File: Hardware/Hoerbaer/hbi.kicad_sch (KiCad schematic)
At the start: 50 parts, among them J10 LEDS, J11 LEDS, J6 BUTTONS, J7 BUTTONS, J8 BUTTONS, J9 LEDS, U2 PCF8574APWR, U3 PCF8574APWR, U4 PCF8574APWR, U5 TLC59108xPW, U6 TLC59108xPW, U7 TLC59108xPW

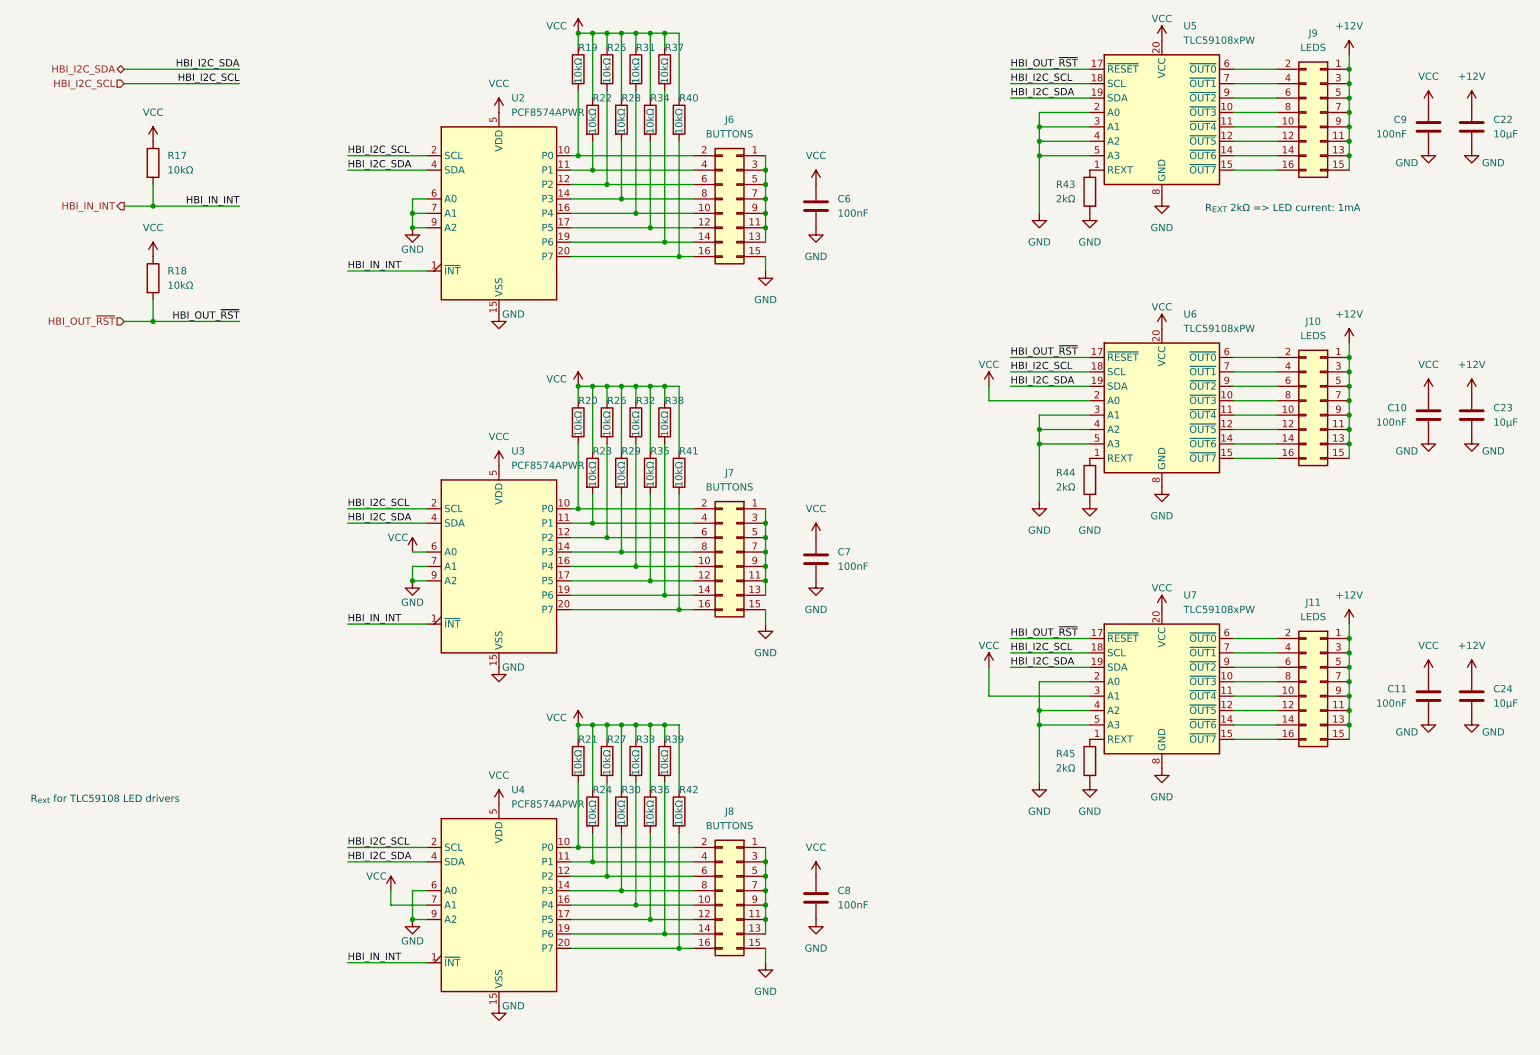
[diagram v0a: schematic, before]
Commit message: Layout drc error free
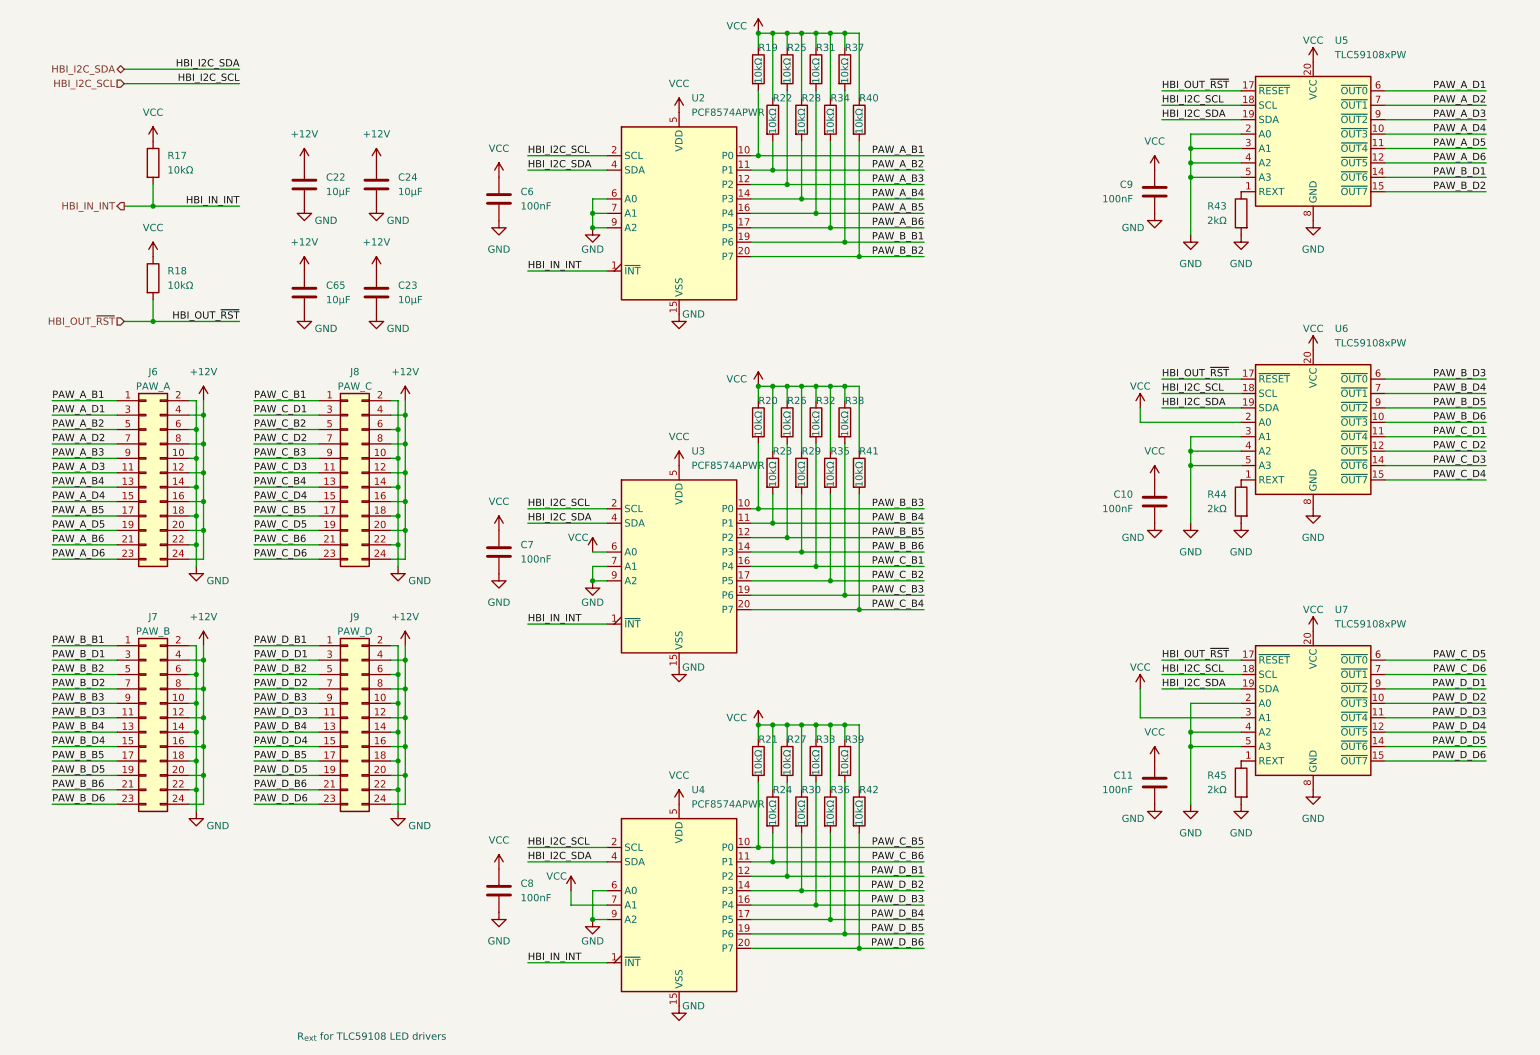
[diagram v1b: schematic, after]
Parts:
- removed J10, J11, J9: LEDS, Connector_PinHeader_2.54mm:PinHeader_2x08_P2.54mm_Vertical, symbol Connector_Generic:Conn_02x08_Odd_Even
- removed J7, J8: BUTTONS, Connector_PinHeader_2.54mm:PinHeader_2x08_P2.54mm_Vertical, symbol Connector_Generic:Conn_02x08_Odd_Even
- added C65: 10µF, Capacitor_SMD:C_0805_2012Metric, symbol Device:C
- added J7: PAW_B, Connector_PinHeader_2.54mm:PinHeader_2x12_P2.54mm_Vertical, symbol Connector_Generic:Conn_02x12_Odd_Even
- added J8: PAW_C, Connector_PinHeader_2.54mm:PinHeader_2x12_P2.54mm_Vertical, symbol Connector_Generic:Conn_02x12_Odd_Even
- added J9: PAW_D, Connector_PinHeader_2.54mm:PinHeader_2x12_P2.54mm_Vertical, symbol Connector_Generic:Conn_02x12_Odd_Even
- J6: value BUTTONS -> PAW_A; footprint Connector_PinHeader_2.54mm:PinHeader_2x08_P2.54mm_Vertical -> Connector_PinHeader_2.54mm:PinHeader_2x12_P2.54mm_Vertical; symbol Connector_Generic:Conn_02x08_Odd_Even -> Connector_Generic:Conn_02x12_Odd_Even
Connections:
- net +12V: now also J6.12 (Pin_12), J6.16 (Pin_16), J6.20 (Pin_20), J6.24 (Pin_24), J6.4 (Pin_4), J6.8 (Pin_8), C65.1, J7.12 (Pin_12), J7.16 (Pin_16), J7.20 (Pin_20), J7.24 (Pin_24), J7.4 (Pin_4), J7.8 (Pin_8), J8.12 (Pin_12), J8.16 (Pin_16), J8.20 (Pin_20), J8.24 (Pin_24), J8.4 (Pin_4), J8.8 (Pin_8), J9.12 (Pin_12), J9.16 (Pin_16), J9.20 (Pin_20), J9.24 (Pin_24), J9.4 (Pin_4), J9.8 (Pin_8)
- net GND: now also J6.10 (Pin_10), J6.14 (Pin_14), J6.18 (Pin_18), J6.2 (Pin_2), J6.22 (Pin_22), J6.6 (Pin_6), C65.2, J7.10 (Pin_10), J7.14 (Pin_14), J7.18 (Pin_18), J7.2 (Pin_2), J7.22 (Pin_22), J7.6 (Pin_6), J8.10 (Pin_10), J8.14 (Pin_14), J8.18 (Pin_18), J8.2 (Pin_2), J8.22 (Pin_22), J8.6 (Pin_6), J9.10 (Pin_10), J9.14 (Pin_14), J9.18 (Pin_18), J9.2 (Pin_2), J9.22 (Pin_22), J9.6 (Pin_6); no longer J6.15 (Pin_15)
- net PAW_C_B6: now reaches R24.2, U4.11 (P1)
- net PAW_C_B6: now also J8.21 (Pin_21)
- net PAW_A_B1: now reaches R19.2, U2.10 (P0)
- net PAW_A_B1: now also J6.1 (Pin_1); no longer J6.2 (Pin_2)
- net PAW_B_B6: now reaches R29.2, U3.14 (P3)
- net PAW_B_B6: now also J7.21 (Pin_21)
- net PAW_C_B5: now reaches R21.2, U4.10 (P0)
- net PAW_C_B5: now also J8.17 (Pin_17)
- net PAW_D_B1: now reaches R27.2, U4.12 (P2)
- net PAW_D_B1: now also J9.1 (Pin_1)
- net PAW_D_B2: now reaches R30.2, U4.14 (P3)
- net PAW_D_B2: now also J9.5 (Pin_5)
- net PAW_D_B3: now reaches R33.2, U4.16 (P4)
- net PAW_D_B3: now also J9.9 (Pin_9)
- net PAW_D_B4: now reaches R36.2, U4.17 (P5)
- net PAW_D_B4: now also J9.13 (Pin_13)
- net PAW_D_B5: now reaches R39.2, U4.19 (P6)
- net PAW_D_B5: now also J9.17 (Pin_17)
- net PAW_D_B6: now reaches R42.2, U4.20 (P7)
- net PAW_D_B6: now also J9.21 (Pin_21)
- net PAW_B_B3: now reaches R20.2, U3.10 (P0)
- net PAW_B_B3: now also J7.9 (Pin_9)
- net PAW_B_B4: now reaches R23.2, U3.11 (P1)
- net PAW_B_B4: now also J7.13 (Pin_13)
- net PAW_B_B5: now reaches R26.2, U3.12 (P2)
- net PAW_B_B5: now also J7.17 (Pin_17)
- net PAW_C_B1: now reaches R32.2, U3.16 (P4)
- net PAW_C_B1: now also J8.1 (Pin_1)
- net PAW_C_B2: now reaches R35.2, U3.17 (P5)
- net PAW_C_B2: now also J8.5 (Pin_5)
- net PAW_C_B3: now reaches R38.2, U3.19 (P6)
- net PAW_C_B3: now also J8.9 (Pin_9)
- net PAW_C_B4: now reaches R41.2, U3.20 (P7)
- net PAW_C_B4: now also J8.13 (Pin_13)
- net PAW_A_B3: now reaches R25.2, U2.12 (P2)
- net PAW_A_B3: now also J6.9 (Pin_9); no longer J6.6 (Pin_6)
- net PAW_D_D2: now reaches U7.10 (~{OUT3})
- net PAW_D_D2: now also J9.7 (Pin_7)
- net PAW_D_D3: now reaches U7.11 (~{OUT4})
- net PAW_D_D3: now also J9.11 (Pin_11)
- net PAW_D_D4: now reaches U7.12 (~{OUT5})
- net PAW_D_D4: now also J9.15 (Pin_15)
- net PAW_D_D5: now reaches U7.14 (~{OUT6})
- net PAW_D_D5: now also J9.19 (Pin_19)
- net PAW_D_D6: now reaches U7.15 (~{OUT7})
- net PAW_D_D6: now also J9.23 (Pin_23)
- net PAW_C_D5: now reaches U7.6 (~{OUT0})
- net PAW_C_D5: now also J8.19 (Pin_19)
- net PAW_C_D6: now reaches U7.7 (~{OUT1})
- net PAW_C_D6: now also J8.23 (Pin_23)
- net PAW_D_D1: now reaches U7.9 (~{OUT2})
- net PAW_D_D1: now also J9.3 (Pin_3)
- net PAW_A_B6: now reaches R34.2, U2.17 (P5)
- net PAW_A_B6: now also J6.21 (Pin_21); no longer J6.12 (Pin_12)
- net PAW_A_B5: now reaches R31.2, U2.16 (P4)
- net PAW_A_B5: now also J6.17 (Pin_17); no longer J6.10 (Pin_10)
- net PAW_B_B1: now reaches R37.2, U2.19 (P6)
- net PAW_B_B1: now also J7.1 (Pin_1); no longer J6.14 (Pin_14)
- net PAW_B_B2: now reaches R40.2, U2.20 (P7)
- net PAW_B_B2: now also J7.5 (Pin_5); no longer J6.16 (Pin_16)
- net PAW_A_B2: now reaches R22.2, U2.11 (P1)
- net PAW_A_B2: now also J6.5 (Pin_5); no longer J6.4 (Pin_4)
- net PAW_A_B4: now reaches R28.2, U2.14 (P3)
- net PAW_A_B4: now also J6.13 (Pin_13); no longer J6.8 (Pin_8)
- net PAW_A_D4: now reaches U5.10 (~{OUT3})
- net PAW_A_D4: now also J6.15 (Pin_15)
- net PAW_A_D5: now reaches U5.11 (~{OUT4})
- net PAW_A_D5: now also J6.19 (Pin_19)
- net PAW_A_D6: now reaches U5.12 (~{OUT5})
- net PAW_A_D6: now also J6.23 (Pin_23)
- net PAW_B_D1: now reaches U5.14 (~{OUT6})
- net PAW_B_D1: now also J7.3 (Pin_3)
- net PAW_B_D2: now reaches U5.15 (~{OUT7})
- net PAW_B_D2: now also J7.7 (Pin_7)
- net PAW_A_D1: now reaches U5.6 (~{OUT0})
- net PAW_A_D1: now also J6.3 (Pin_3)
- net PAW_A_D2: now reaches U5.7 (~{OUT1})
- net PAW_A_D2: now also J6.7 (Pin_7)
- net PAW_A_D3: now reaches U5.9 (~{OUT2})
- net PAW_A_D3: now also J6.11 (Pin_11)
- net PAW_B_D6: now reaches U6.10 (~{OUT3})
- net PAW_B_D6: now also J7.23 (Pin_23)
- net PAW_C_D1: now reaches U6.11 (~{OUT4})
- net PAW_C_D1: now also J8.3 (Pin_3)
- net PAW_C_D2: now reaches U6.12 (~{OUT5})
- net PAW_C_D2: now also J8.7 (Pin_7)
- net PAW_C_D3: now reaches U6.14 (~{OUT6})
- net PAW_C_D3: now also J8.11 (Pin_11)
- net PAW_C_D4: now reaches U6.15 (~{OUT7})
- net PAW_C_D4: now also J8.15 (Pin_15)
- net PAW_B_D3: now reaches U6.6 (~{OUT0})
- net PAW_B_D3: now also J7.11 (Pin_11)
- net PAW_B_D4: now reaches U6.7 (~{OUT1})
- net PAW_B_D4: now also J7.15 (Pin_15)
- net PAW_B_D5: now reaches U6.9 (~{OUT2})
- net PAW_B_D5: now also J7.19 (Pin_19)
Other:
- note removed: "R_{EXT} 2kΩ => LED current: 1mA"
- moved on the sheet: C10, C11, C22, C23, C24, C6, C7, C8, C9, R19, R20, R21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

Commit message: Order numbers
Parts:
- C10, C11, C6, C7, C8, C9: JLCPCB (none) -> C458949; MPN (none) -> MT15B104K160CT
- U6, U7: JLCPCB (none) -> C130031; MPN (none) -> TLC59108IPWR
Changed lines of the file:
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@@
+      (effects (font (size 1.27 1.27)) hide)
+    )
+    (property "JLCPCB" "C458949" (at 99.06 110.49 0)
+      (effects (font (size 1.27 1.27)) hide)
+    )
+    (property "MPN" "MT15B104K160CT" (at 99.06 110.49 0)
       (effects (font (size 1.27 1.27)) hide)
     )
@@
       (effects (font (size 1.27 1.27)) hide)
     )
+    (property "JLCPCB" "C130031" (at 242.57 139.7 0)
+      (effects (font (size 1.27 1.27)) hide)
+    )
+    (property "MPN" "TLC59108IPWR" (at 242.57 139.7 0)
+      (effects (font (size 1.27 1.27)) hide)
+    )
     (pin "1")
     (pin "10")
@@
       (effects (font (size 1.27 1.27)) hide)
     )
+    (property "JLCPCB" "C458949" (at 214.63 46.99 0)
+      (effects (font (size 1.27 1.27)) hide)
+    )
+    (property "MPN" "MT15B104K160CT" (at 214.63 46.99 0)
+      (effects (font (size 1.27 1.27)) hide)
+    )
     (pin "1")
     (pin "2")
@@
       (effects (font (size 1.27 1.27)) hide)
     )
+    (property "JLCPCB" "C458949" (at 99.06 48.26 0)
+      (effects (font (size 1.27 1.27)) hide)
+    )
+    (property "MPN" "MT15B104K160CT" (at 99.06 48.26 0)
+      (effects (font (size 1.27 1.27)) hide)
+    )
     (pin "1")
     (pin "2")
@@
       (effects (font (size 1.27 1.27)) hide)
     )
+    (property "JLCPCB" "C458949" (at 214.63 151.13 0)
+      (effects (font (size 1.27 1.27)) hide)
+    )
+    (property "MPN" "MT15B104K160CT" (at 214.63 151.13 0)
+      (effects (font (size 1.27 1.27)) hide)
+    )
     (pin "1")
     (pin "2")
@@
     )
     (property "Datasheet" "~" (at 99.06 170.18 0)
+      (effects (font (size 1.27 1.27)) hide)
+    )
+    (property "JLCPCB" "C458949" (at 99.06 170.18 0)
+      (effects (font (size 1.27 1.27)) hide)
+    )
+    (property "MPN" "MT15B104K160CT" (at 99.06 170.18 0)
       (effects (font (size 1.27 1.27)) hide)
     )
@@
       (effects (font (size 1.27 1.27)) hide)
     )
+    (property "JLCPCB" "C130031" (at 242.57 90.17 0)
+      (effects (font (size 1.27 1.27)) hide)
+    )
+    (property "MPN" "TLC59108IPWR" (at 242.57 90.17 0)
+      (effects (font (size 1.27 1.27)) hide)
+    )
     (pin "1")
     (pin "10")
@@
       (effects (font (size 1.27 1.27)) hide)
     )
+    (property "JLCPCB" "C458949" (at 214.63 101.6 0)
+      (effects (font (size 1.27 1.27)) hide)
+    )
+    (property "MPN" "MT15B104K160CT" (at 214.63 101.6 0)
+      (effects (font (size 1.27 1.27)) hide)
+    )
